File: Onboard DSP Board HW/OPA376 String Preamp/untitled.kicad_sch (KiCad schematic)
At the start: 13 parts, among them J1 Input, U1 OPA376AIDCKT

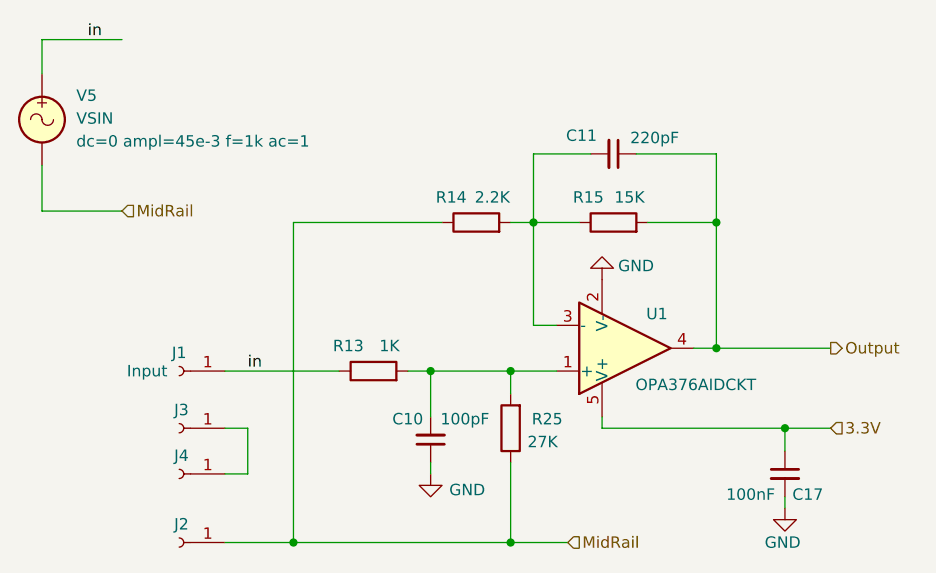
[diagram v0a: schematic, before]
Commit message: WIP
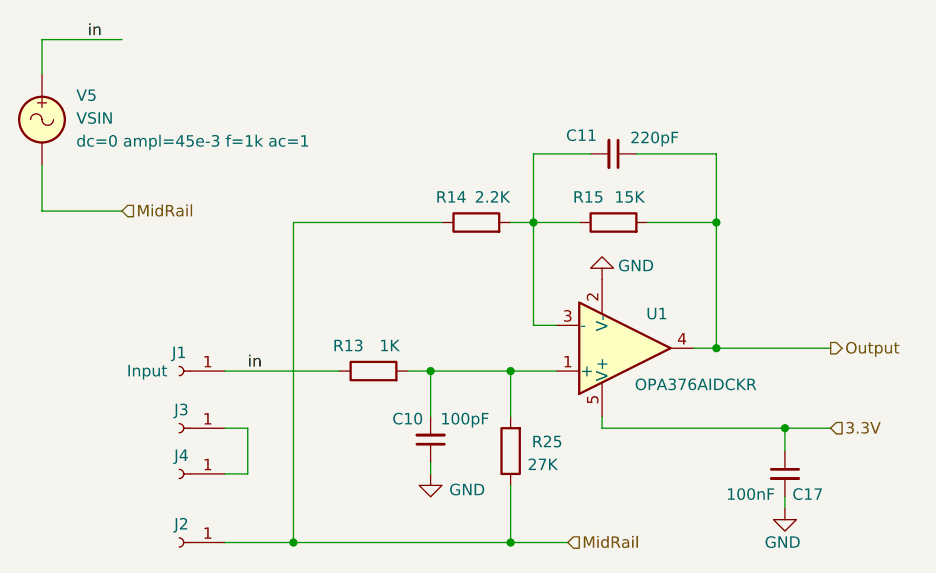
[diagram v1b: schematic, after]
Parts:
- U1: value OPA376AIDCKT -> OPA376AIDCKR
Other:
- moved on the sheet: R25
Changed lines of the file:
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@@
 	(paper "A4")
+	(junction
+		(at 165.1 87.63)
+		(diameter 0)
+		(color 0 0 0 0)
+	)
+	(junction
+		(at 187.96 66.04)
+		(diameter 0)
+		(color 0 0 0 0)
+	)
 	(junction
 		(at 165.1 68.58)
@@
 	)
 	(junction
-		(at 165.1 87.63)
-		(diameter 0)
-		(color 0 0 0 0)
-	)
-	(junction
-		(at 187.96 66.04)
-		(diameter 0)
-		(color 0 0 0 0)
-	)
-	(junction
 		(at 167.64 52.07)
 		(diameter 0)
@@
 	(wire
 		(pts
-			(xy 165.1 68.58) (xy 165.1 71.12)
+			(xy 165.1 68.58) (xy 165.1 73.66)
 		)
 		(stroke
@@
 	(wire
 		(pts
-			(xy 165.1 78.74) (xy 165.1 87.63)
+			(xy 165.1 81.28) (xy 165.1 87.63)
 		)
 		(stroke
@@
 	(symbol
 		(lib_id "Device:R")
-		(at 165.1 74.93 180)
+		(at 165.1 77.47 180)
 		(unit 1)
 		(body_style 1)
@@
 		(dnp no)
 		(property "Reference" "R25"
-			(at 169.164 73.914 0)
+			(at 169.164 76.454 0)
 			(show_name no)
 			(do_not_autoplace no)
@@
 		)
 		(property "Value" "27K"
-			(at 168.656 76.454 0)
+			(at 168.656 78.994 0)
 			(show_name no)
 			(do_not_autoplace no)
@@
 		)
 		(property "Footprint" "Resistor_SMD:R_0402_1005Metric"
-			(at 166.878 74.93 90)
+			(at 166.878 77.47 90)
 			(hide yes)
 			(show_name no)
@@
 		)
 		(property "Datasheet" ""
-			(at 165.1 74.93 0)
+			(at 165.1 77.47 0)
 			(hide yes)
 			(show_name no)
@@
 		)
 		(property "Description" "Resistor"
-			(at 165.1 74.93 0)
+			(at 165.1 77.47 0)
 			(hide yes)
 			(show_name no)
@@
 			)
 		)
-		(property "Value" "OPA376AIDCKT"
+		(property "Value" "OPA376AIDCKR"
 			(at 185.674 70.104 0)
 			(show_name no)
